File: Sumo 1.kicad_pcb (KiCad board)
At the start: 2 copper layers, 58.4 x 43.2 mm, 23 parts, among them J1 DIST SENS, J2 LEFT SENS, J3 RIGHT SENS, J4 Trinket Pro 5V, M1 Logic Power, M2 Motor Power, M3 Motor1, M4 Motor2, U1 TB6612FNG

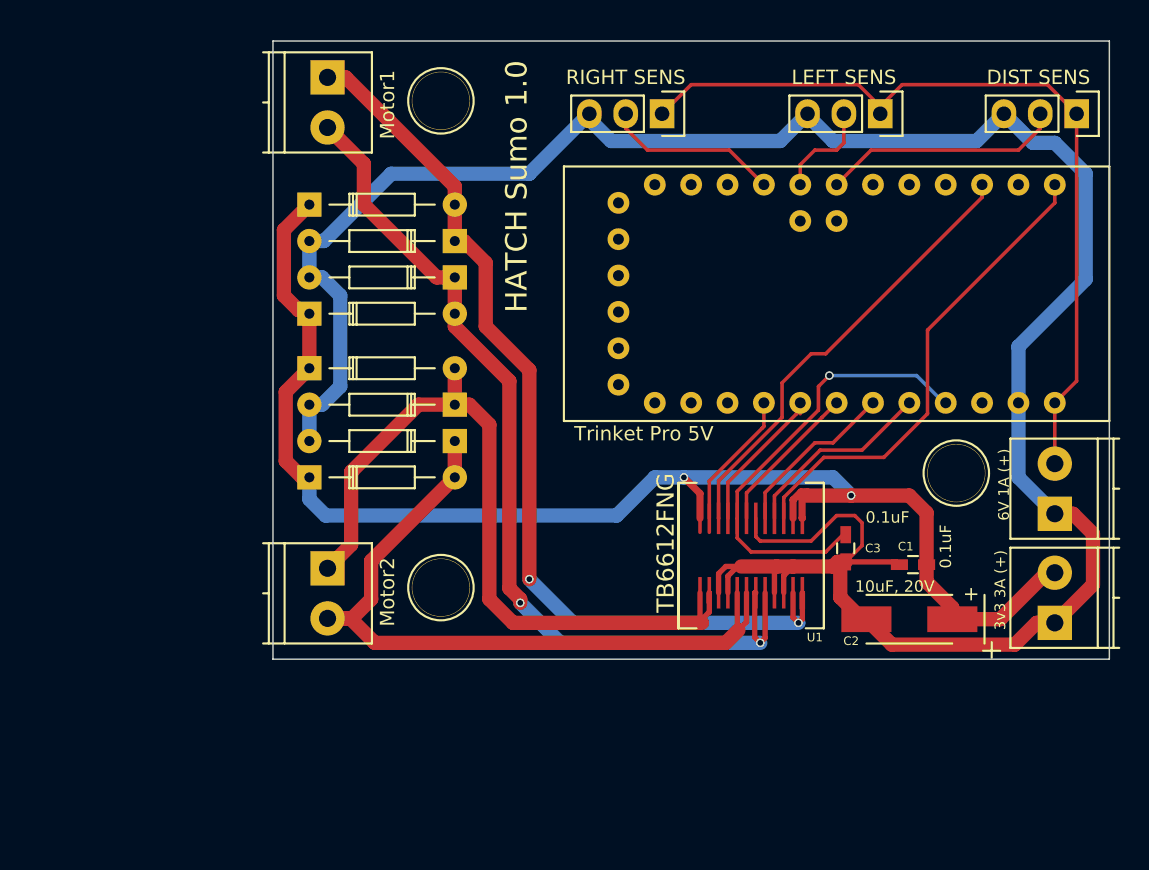
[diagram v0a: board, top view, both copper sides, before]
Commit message: New spin!
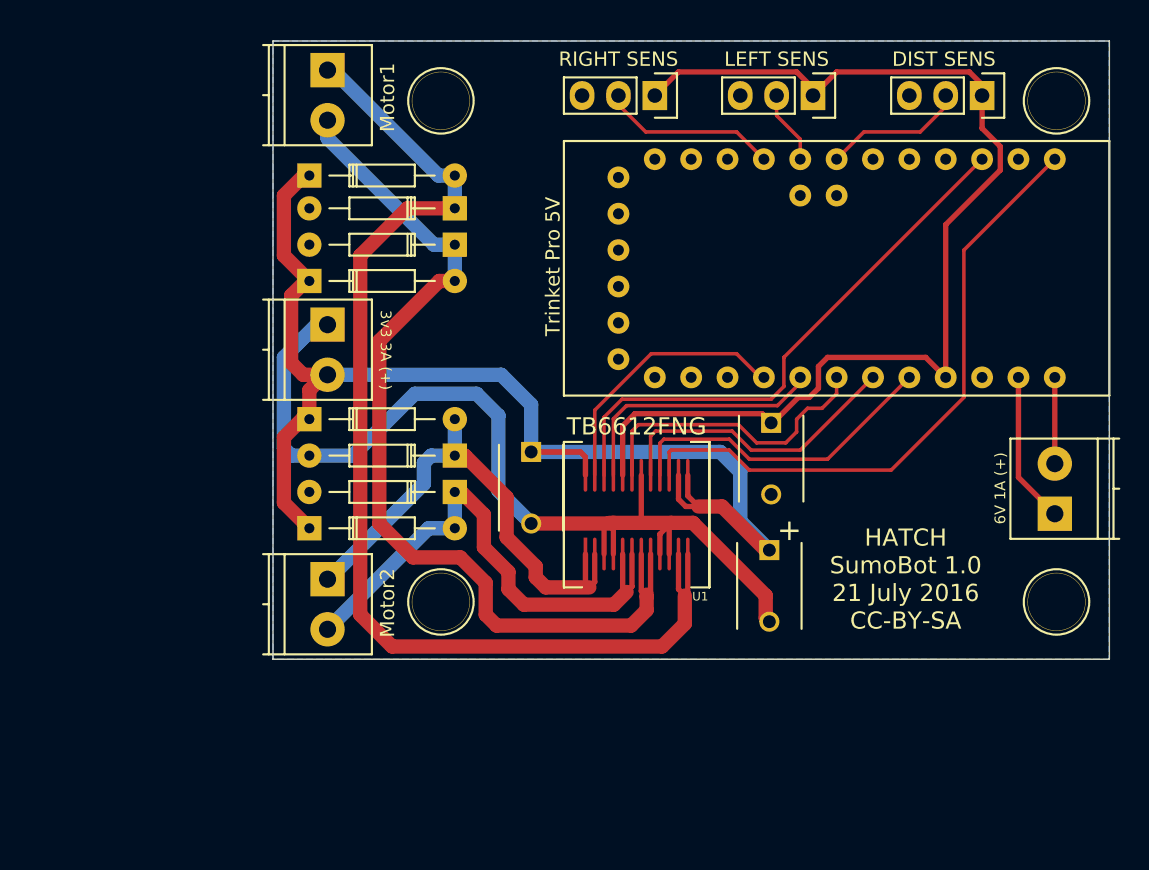
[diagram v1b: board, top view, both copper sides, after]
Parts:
- added ?: , Diodes_ThroughHole:Diode_DO-35_SOD27_Horizontal_RM10, B.Cu at (141.0, 115.3)
- added ?: , Diodes_ThroughHole:Diode_DO-35_SOD27_Horizontal_RM10, B.Cu at (130.8, 117.9)
- added ?: , Diodes_ThroughHole:Diode_DO-35_SOD27_Horizontal_RM10, B.Cu at (141.0, 112.8)
- added ?: , Diodes_ThroughHole:Diode_DO-35_SOD27_Horizontal_RM10, B.Cu at (141.0, 98.0)
- added ?: , Diodes_ThroughHole:Diode_DO-35_SOD27_Horizontal_RM10, B.Cu at (130.8, 110.2)
- added ?: , Diodes_ThroughHole:Diode_DO-35_SOD27_Horizontal_RM10, B.Cu at (130.8, 100.6)
- added ?: , Diodes_ThroughHole:Diode_DO-35_SOD27_Horizontal_RM10, B.Cu at (141.0, 95.5)
- added ?: , Diodes_ThroughHole:Diode_DO-35_SOD27_Horizontal_RM10, B.Cu at (130.8, 93.2)
- added ?: , Connect:1pin, F.Cu at (183.0, 88.0)
- C1, C3: footprint Capacitors_SMD:C_0603_HandSoldering -> Capacitors_ThroughHole:C_Disc_D6_P5
- C2: footprint Capacitors_Tantalum_SMD:TantalC_SizeC_EIA-6032_HandSoldering -> Capacitors_ThroughHole:C_Disc_D6_P5
- moved M2 54.9 mm to (132.1, 103.6), turned to 270 degrees
- moved C1 27.8 mm to (146.3, 112.5), turned to 270 degrees
- moved ? 11.4 mm to (183.0, 123.0)
- moved C2 10.9 mm to (162.9, 119.4), turned to 270 degrees
- moved C3 10.2 mm to (163.1, 110.5)
- moved U1 8.50 mm to (153.7, 116.9)
- moved J1 6.73 mm to (177.8, 87.6)
- moved J2 4.87 mm to (166.0, 87.6)
- moved D5 3.56 mm to (130.8, 110.2)
- moved D6 3.56 mm to (141.0, 112.8)
- moved D7 3.56 mm to (130.8, 117.9)
- moved D8 3.56 mm to (141.0, 115.3)
- moved D2 2.29 mm to (141.0, 95.5)
- moved D3 2.29 mm to (130.8, 100.6)
- moved D4 2.29 mm to (141.0, 98.0)
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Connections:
- J1 pad 1: +6V -> /V_LOGIC
- J2 pad 1: +6V -> /V_LOGIC
- J3 pad 1: +6V -> /V_LOGIC
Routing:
- net GND: track 171.1 -> 80.9 mm
- net +6V: track 57.5 -> 6.03 mm
- net /V_LOGIC: track 31.4 -> 78.1 mm, vias 1 -> 0
- net /A01_W: track 55.1 -> 36.3 mm
- net /A02_W: track 52.5 -> 37.6 mm
- net /B01_W: track 67.6 -> 79.6 mm, vias 2 -> 0
- net /STBY_W: track 10.7 -> 22.2 mm
- net /PWMB_W: track 33.6 -> 44.2 mm
- net /BIN1_W: track 11.9 -> 21.1 mm
- net /BIN2_W: track 13.7 -> 22.7 mm
- net /PWMA_W: track 9.65 -> 18.7 mm
- net +3V3: track 98.0 -> 89.6 mm, vias 2 -> 0
- net /AIN2_W: track 31.5 -> 39.1 mm
- net /AIN1_W: track 11.3 -> 18.4 mm
- net /DIST_SIGNAL: track 16.9 -> 10.5 mm
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- added copper zone on B.Cu, net GND
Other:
- board text added: "+"
- board text added: "HATCH SumoBot 1.0 21 July 2016 CC-BY-SA"
- board text removed: "HATCH Sumo 1.0"

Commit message: Sumo v1 files
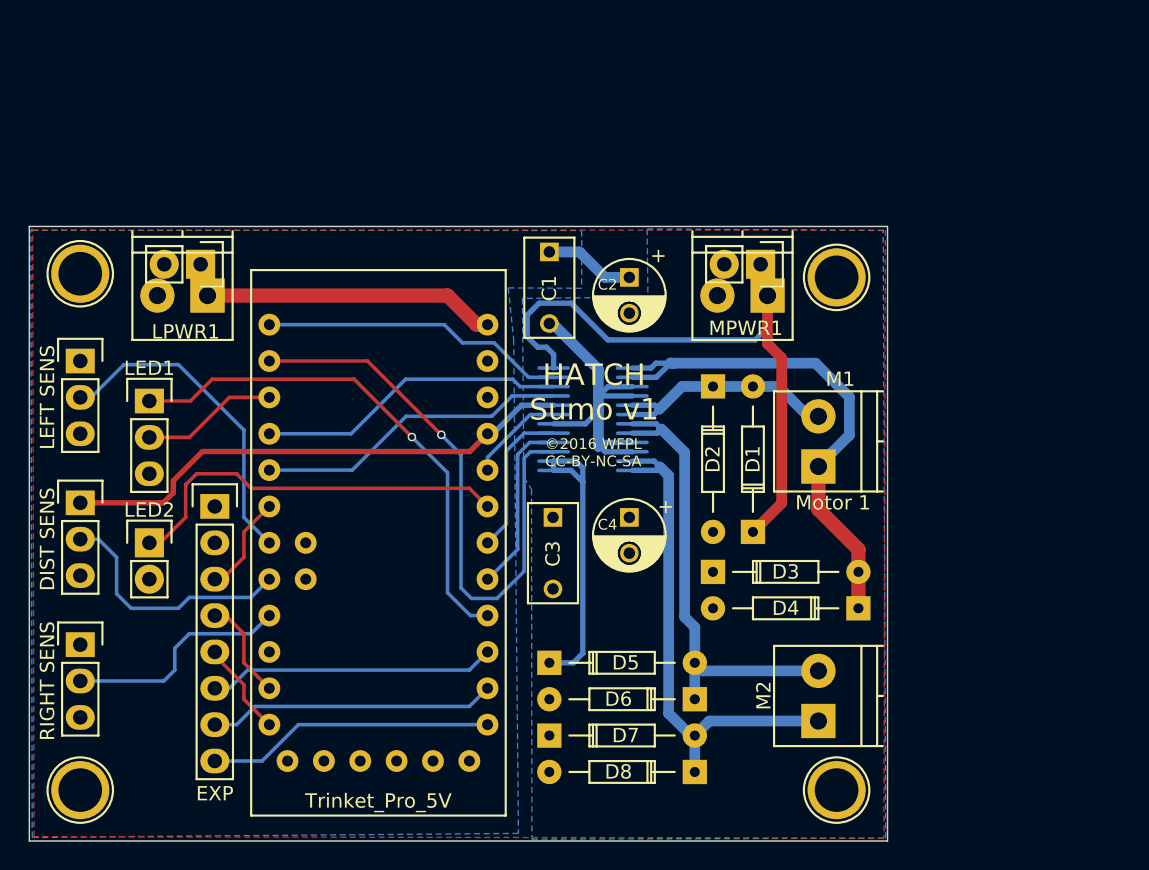
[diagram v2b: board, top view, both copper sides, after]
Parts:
- removed the ? at (141.0, 115.3)
- removed the ? at (140.0, 123.0)
- removed the ? at (183.0, 123.0)
- removed the ? at (140.0, 88.0)
- removed the ? at (130.8, 117.9)
- removed the ? at (141.0, 112.8)
- removed the ? at (141.0, 98.0)
- removed the ? at (130.8, 110.2)
- removed the ? at (130.8, 100.6)
- removed the ? at (141.0, 95.5)
- removed the ? at (130.8, 93.2)
- removed the ? at (183.0, 88.0)
- removed the C1 at (146.3, 112.5)
- removed the C2 at (162.9, 119.4)
- removed the C3 at (163.1, 110.5)
- removed the D1 at (130.8, 93.2)
- removed the D2 at (141.0, 95.5)
- removed the D3 at (130.8, 100.6)
- removed the D4 at (141.0, 98.0)
- removed the D5 at (130.8, 110.2)
- removed the D6 at (141.0, 112.8)
- removed the D7 at (130.8, 117.9)
- removed the D8 at (141.0, 115.3)
- removed J2: LEFT SENS, Pin_Headers:Pin_Header_Straight_1x03
- removed J3: RIGHT SENS, Pin_Headers:Pin_Header_Straight_1x03
- removed J4: Trinket Pro 5V, ArduinoFootprints:Trinket_Pro_5V
- removed the M1 at (182.9, 116.8)
- removed the M2 at (132.1, 103.6)
- removed M3: Motor1, Terminal_Blocks:TerminalBlock_Pheonix_PT-3.5mm_2pol
- removed M4: Motor2, Terminal_Blocks:TerminalBlock_Pheonix_PT-3.5mm_2pol
- added ?: , Connect:1pin, F.Cu at (114.8, 136.1)
- added ?: , Pin_Headers:Pin_Header_Straight_1x02, F.Cu at (162.3, 99.4)
- added ?: , Connect:1pin, F.Cu at (114.8, 100.1)
- added ?: DIST SENS, Pin_Headers:Pin_Header_Straight_1x03, F.Cu at (114.8, 116.1)
- added ?: LEFT SENS, Pin_Headers:Pin_Header_Straight_1x03, F.Cu at (114.8, 106.2)
- added ?: RIGHT SENS, Pin_Headers:Pin_Header_Straight_1x03, F.Cu at (114.8, 126.0)
- added ?: LED1, Pin_Headers:Pin_Header_Straight_1x03, F.Cu at (119.6, 109.0)
- added ?: LED2, Pin_Headers:Pin_Header_Straight_1x02, F.Cu at (119.6, 118.9)
- added ?: , Connect:1pin, F.Cu at (167.6, 100.3)
- added ?: , Pin_Headers:Pin_Header_Straight_1x02, F.Cu at (123.2, 99.4)
- added C1: 0.1uF, Capacitors_ThroughHole:C_Rect_L7_W3.5_P5, B.Cu at (147.6, 103.6)
- added C1: , Capacitors_ThroughHole:C_Rect_L7_W3.5_P5, F.Cu at (147.6, 98.6)
- added C2: 10uF, 20V, Capacitors_ThroughHole:C_Radial_D5_L6_P2.5, B.Cu at (153.2, 100.3)
- added C2: , Capacitors_ThroughHole:C_Radial_D5_L6_P2.5, F.Cu at (153.2, 100.3)
- added C3: 0.1uF, Capacitors_ThroughHole:C_Rect_L7_W3.5_P5, B.Cu at (147.8, 122.2)
- added C3: , Capacitors_ThroughHole:C_Rect_L7_W3.5_P5, F.Cu at (147.8, 117.1)
- added C4: 10uF, 20V, Capacitors_ThroughHole:C_Radial_D5_L6_P2.5, B.Cu at (153.2, 117.1)
- added C4: , Capacitors_ThroughHole:C_Radial_D5_L6_P2.5, F.Cu at (153.2, 117.1)
- added D1: , Diodes_ThroughHole:Diode_DO-35_SOD27_Horizontal_RM10, B.Cu at (161.8, 118.1)
- added D1: , Diodes_ThroughHole:Diode_DO-35_SOD27_Horizontal_RM10, F.Cu at (161.8, 118.1)
- added D2: , Diodes_ThroughHole:Diode_DO-35_SOD27_Horizontal_RM10, B.Cu at (159.0, 108.0)
- added D2: , Diodes_ThroughHole:Diode_DO-35_SOD27_Horizontal_RM10, F.Cu at (159.0, 108.0)
- added D3: , Diodes_ThroughHole:Diode_DO-35_SOD27_Horizontal_RM10, B.Cu at (159.0, 120.9)
- added D3: , Diodes_ThroughHole:Diode_DO-35_SOD27_Horizontal_RM10, F.Cu at (159.0, 120.9)
- added D4: , Diodes_ThroughHole:Diode_DO-35_SOD27_Horizontal_RM10, B.Cu at (169.2, 123.4)
- added D4: , Diodes_ThroughHole:Diode_DO-35_SOD27_Horizontal_RM10, F.Cu at (169.2, 123.4)
- added D5: , Diodes_ThroughHole:Diode_DO-35_SOD27_Horizontal_RM10, B.Cu at (147.6, 127.3)
- added D5: , Diodes_ThroughHole:Diode_DO-35_SOD27_Horizontal_RM10, F.Cu at (147.6, 127.3)
- added D6: , Diodes_ThroughHole:Diode_DO-35_SOD27_Horizontal_RM10, B.Cu at (157.7, 129.8)
- added D6: , Diodes_ThroughHole:Diode_DO-35_SOD27_Horizontal_RM10, F.Cu at (157.7, 129.8)
- added D7: , Diodes_ThroughHole:Diode_DO-35_SOD27_Horizontal_RM10, B.Cu at (147.6, 132.3)
- added D7: , Diodes_ThroughHole:Diode_DO-35_SOD27_Horizontal_RM10, F.Cu at (147.6, 132.3)
- added D8: D1-8: 1N4001, Diodes_ThroughHole:Diode_DO-35_SOD27_Horizontal_RM10, B.Cu at (157.7, 134.9)
- added D8: , Diodes_ThroughHole:Diode_DO-35_SOD27_Horizontal_RM10, F.Cu at (157.7, 134.9)
- added EXP: , Pin_Headers:Pin_Header_Straight_1x08, F.Cu at (124.2, 116.3)
- added LPWR1: Logic Power, Terminal_Blocks:TerminalBlock_Pheonix_PT-3.5mm_2pol, B.Cu at (120.1, 101.6)
- added LPWR1: Logic Power, Terminal_Blocks:TerminalBlock_Pheonix_PT-3.5mm_2pol, F.Cu at (123.7, 101.6)
- added M1: Motor1, Terminal_Blocks:TerminalBlock_Pheonix_PT-3.5mm_2pol, B.Cu at (166.4, 110.0)
- added M1: Motor 1, Terminal_Blocks:TerminalBlock_Pheonix_PT-3.5mm_2pol, F.Cu at (166.4, 113.5)
- added M2: , Terminal_Blocks:TerminalBlock_Pheonix_PT-3.5mm_2pol, B.Cu at (166.4, 127.8)
- added M2: Motor 2, Terminal_Blocks:TerminalBlock_Pheonix_PT-3.5mm_2pol, F.Cu at (166.4, 131.3)
- added MPWR1: Motor Power, Terminal_Blocks:TerminalBlock_Pheonix_PT-3.5mm_2pol, B.Cu at (159.3, 101.6)
- added MPWR1: Motor Pwr, Terminal_Blocks:TerminalBlock_Pheonix_PT-3.5mm_2pol, F.Cu at (162.8, 101.6)
- added P1: , Pin_Headers:Pin_Header_Straight_1x03, B.Cu at (114.8, 116.1)
- added P2: , Pin_Headers:Pin_Header_Straight_1x03, B.Cu at (114.8, 106.2)
- added P3: , Pin_Headers:Pin_Header_Straight_1x03, B.Cu at (114.8, 126.0)
- added P4: , Pin_Headers:Pin_Header_Straight_1x03, B.Cu at (119.6, 109.0)
- added P5: , Pin_Headers:Pin_Header_Straight_1x02, B.Cu at (119.6, 118.9)
- added REF**: 1pin, Connect:1pin, F.Cu at (167.6, 136.1)
- added XP1: EXP, Pin_Headers:Pin_Header_Straight_1x08, B.Cu at (124.2, 116.3)
- J1: value DIST SENS -> Trinket_Pro_5V; footprint Pin_Headers:Pin_Header_Straight_1x03 -> ArduinoFootprints:Trinket_Pro_5V
- U1: moved to B.Cu
- moved J1 52.5 mm to (126.7, 99.8), turned to 0 degrees
- moved U1 7.33 mm to (150.6, 110.2), turned to 270 degrees
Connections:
- net +3V3 renamed V_MOTOR
- net /A01_W renamed A01
- net /A02_W renamed A02
- net /B01_W renamed B01
- net /B02_W renamed B02
- J1 pad 1: /V_LOGIC -> RST
- J1 pad 3: GND -> LED1_RED
- U1 pad 10: GND -> GND_LOGIC
- U1 pad 15: /PWMB_W -> PWMB
- U1 pad 16: /BIN2_W -> BIN2
- U1 pad 17: /BIN1_W -> BIN1
- U1 pad 18: GND -> GND_LOGIC
- U1 pad 19: /STBY_W -> STBY
- U1 pad 20: /V_LOGIC -> V_LOGIC
- U1 pad 21: /AIN1_W -> AIN1
- U1 pad 22: /AIN2_W -> AIN2
- U1 pad 23: /PWMA_W -> PWMA
- U1 pad 3: GND -> GND_LOGIC
- U1 pad 4: GND -> GND_LOGIC
- U1 pad 9: GND -> GND_LOGIC
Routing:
- net GND: track 80.9 -> 0.00 mm
- net /V_LOGIC: track 78.1 -> 0.00 mm
- net /PWMB_W: track 44.2 -> 0.00 mm
- net B01: track 79.6 -> 36.2 mm
- net V_LOGIC: track 0.00 -> 42.7 mm
- net PWMB: track 0.00 -> 41.1 mm, vias 0 -> 1
- net /AIN2_W: track 39.1 -> 0.00 mm
- net LED1_RED: track 0.00 -> 36.5 mm, vias 0 -> 1
- net B02: track 66.2 -> 33.0 mm
- net LED2: track 0.00 -> 27.9 mm
- net V_MOTOR: track 89.6 -> 64.2 mm
- net GND_LOGIC: track 0.00 -> 23.9 mm
- net SENS_LEFT: track 0.00 -> 22.9 mm
- net /BIN2_W: track 22.7 -> 0.00 mm
- net V_BAT: track 0.00 -> 22.6 mm
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- added copper zone on F.Cu, net GND_LOGIC
- added copper zone on B.Cu, net V_LOGIC
- added copper zone on B.Cu, net V_MOTOR
- removed copper zone on B.Cu, net GND
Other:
- board size 58.4 x 43.2 mm -> 59.9 x 42.9 mm
- net class MotorPower removed
- board text added: "3v3"
- board text added: "5V"
- board text added: "6V"
- board text added: "A4"
- board text added: "A5"
- board text added: "AREF"
- board text added: "D1-8 are 1N4001 or equivalent. Be careful of polarity for C2, C4, and diodes! Smaller power pads are for JST or pin headers; larger for terminal blocks."
- board text added: "DIST"
- board text added: "GND"
- board text added: "GRN"
- board text added: "HATCH Sumo v1"
- board text added: "LEFT"
- board text added: "RED"
- board text added: "RIGHT"
- board text added: "RST"
- board text added: "RX"
- board text added: "TX"
- board text added: "Trinket Pro 5V"
- board text added: "©2016 WFPL CC-BY-NC-SA"
- board text added: "©2016 WFPL CC-BY-NC-SA Logic Power: 6VDC @ 1mA Motor Power: 3.3VDC @ 3A LED1 and 2 can drive 20mA at 5VDC."
- board text removed: "(+)"
- board text removed: "3v3 3A (+)"
- board text removed: "6V 1A (+)"
- board text removed: "HATCH SumoBot 1.0 21 July 2016 CC-BY-SA"
- board text removed: "HATCH Trinket Pro SumoBot v1.0, 21 July 2016 CC-BY-SA"
- board text removed: "Logic Power – 6VDC 1A"
- board text removed: "Motor Power 3.3VDC 3A"
